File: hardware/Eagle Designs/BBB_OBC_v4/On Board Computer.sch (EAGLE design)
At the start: 34 parts, among them J1 MOLEX_503763-0491MOLEX_503763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, J10 503763-0591, J11 503763-0591, J12 503763-0691, J13 MOLEX_503763-0291MOLEX_503763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, J16 U.FL-R-SMT-1(01), J2 MOLEX_503763-0491MOLEX_503763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, J6 MOLEX_503763-0491MOLEX_503763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, J9 U.FL-R-SMT-1(01), P8 SSW-123-02-G-D, P9 SSW-123-02-G-D, U1 TMP36FSZR_8_ADI-L, U2 LTC1477CS8LINEAR_TECHNOLOGY_L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, U3 RFM69HCW_433_900, U6 ORION_A38LORION_A38L, U7 PA1010D, X1 C25582-40G-M36-0A, X2 SSW-120-02-G-D

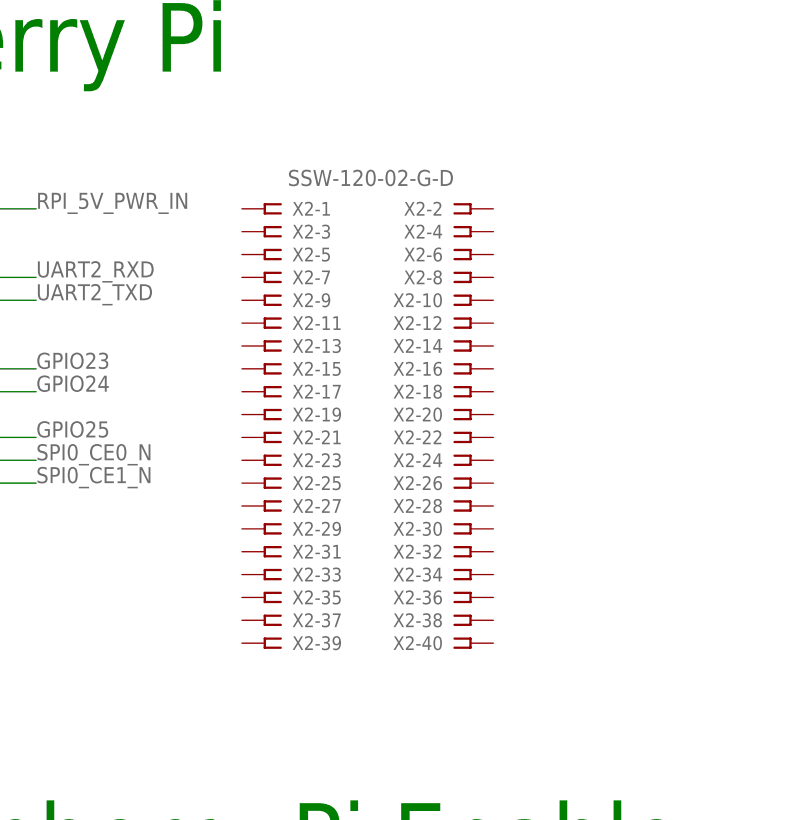
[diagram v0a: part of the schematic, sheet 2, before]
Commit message: OBC v4 edits
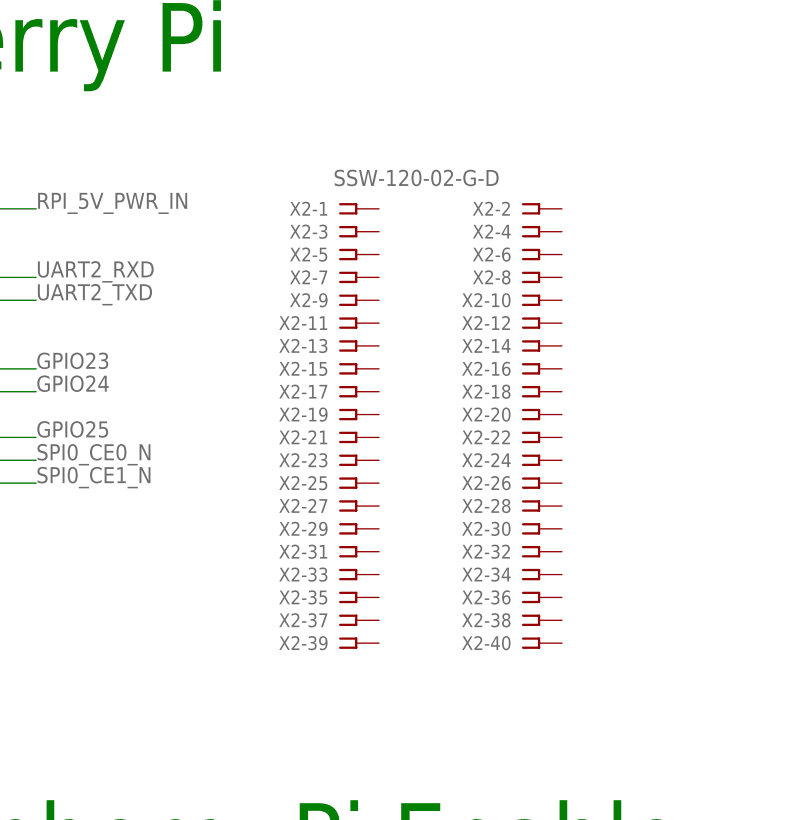
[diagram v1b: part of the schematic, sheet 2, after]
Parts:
- removed 3V3_BUS, GPS_BOOTSEL: (no value), wirepad:1,6/0,9
- removed GND: GND, wirepad:1,6/0,9
- added L1: L, L:L
- added R4, R5, R6: 0, HSFL_Main_Library:RESISTOR0805-RES
- X2: device con-samtec:SSW-120-02-G-D -> con-samtec-edited:SSW-120-02-G-D
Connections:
- removed net GPS_BOOTSEL: GPS_BOOTSEL.P, U6.GPS_BOOTSEL
- new net N$16: R4.2, R5.2, U6.GPS_BOOTSEL
- new net RF_GND: R6.1, U6.GND_RF, U6.P$22, U6.P$24, U6.P$25, U6.P$27, U6.P$28, U6.P$29, U6.P$31, U6.P$33
- net +3V3_VCC: now also L1.1, U6.P$58
- net 3V3_BUS: now also R5.1; no longer 3V3_BUS.P
- net GND: now also R4.1, R6.2, U6.P$10, U6.P$15, U6.P$19; no longer GND.P, U6.GND_RF
- net N$17: now also L1.2
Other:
- moved on the sheet: J9, X2-1, X2-10, X2-11, X2-12, X2-13, X2-14, X2-15, X2-16, X2-17, X2-18, X2-19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
